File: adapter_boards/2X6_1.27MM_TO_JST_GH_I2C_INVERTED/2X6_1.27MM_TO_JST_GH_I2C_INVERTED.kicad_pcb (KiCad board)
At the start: 2 copper layers, 11 x 10.2 mm, 3 parts, among them J1 1.27mm 2x6-PTH, J2 SM04B-GHS-TB

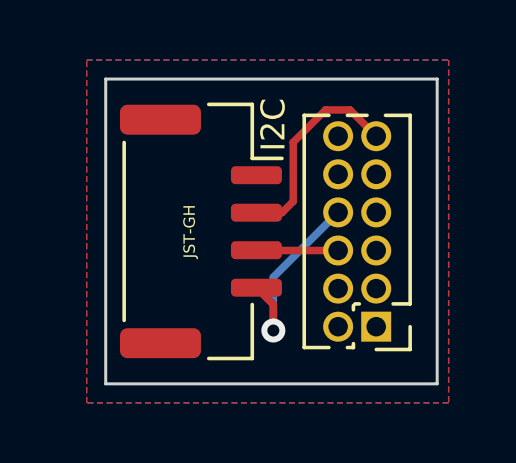
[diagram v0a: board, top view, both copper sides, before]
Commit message: Added optional pullup resistors to I2C JST-GH adapter boards
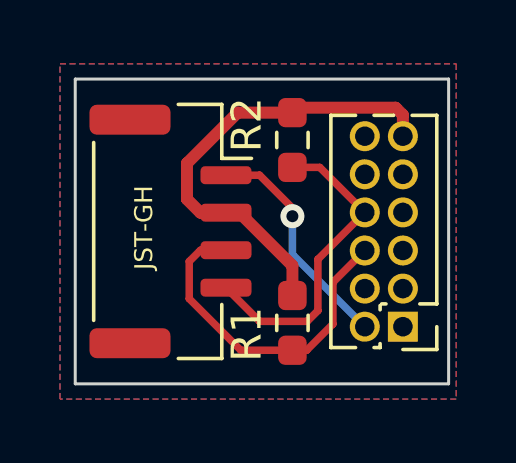
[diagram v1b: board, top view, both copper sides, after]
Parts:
- added R1: 2k, Resistor_SMD:R_0603_1608Metric_Pad0.98x0.95mm_HandSolder, F.Cu at (151.0, 102.1)
- added R2: 2k, Resistor_SMD:R_0603_1608Metric_Pad0.98x0.95mm_HandSolder, F.Cu at (151.0, 96.0)
- moved J2 1.02 mm to (146.9, 99.1)
- moved   0.90 mm to (148.7, 96.3)
- moved J1 0.89 mm to (154.7, 102.2)
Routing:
- net /I2C_SCL: track 2.73 -> 11.4 mm
- net /3V3: track 6.93 -> 15.4 mm
- net /GND: track 0.00 -> 7.62 mm, vias 0 -> 1
- net /I2C_SDA: track 6.49 -> 10.6 mm, vias 1 -> 0
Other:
- board size 11 x 10.2 mm -> 12.4 x 10.2 mm
- board text removed: "I2C"
